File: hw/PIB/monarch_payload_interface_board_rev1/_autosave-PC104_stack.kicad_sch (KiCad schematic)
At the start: 19 parts, among them U1 Payload, U10 AD7124-8BCPZ-RL, U11 WSK06121L000FEA, U12 WSK06121L000FEA, U13 WSK06121L000FEA

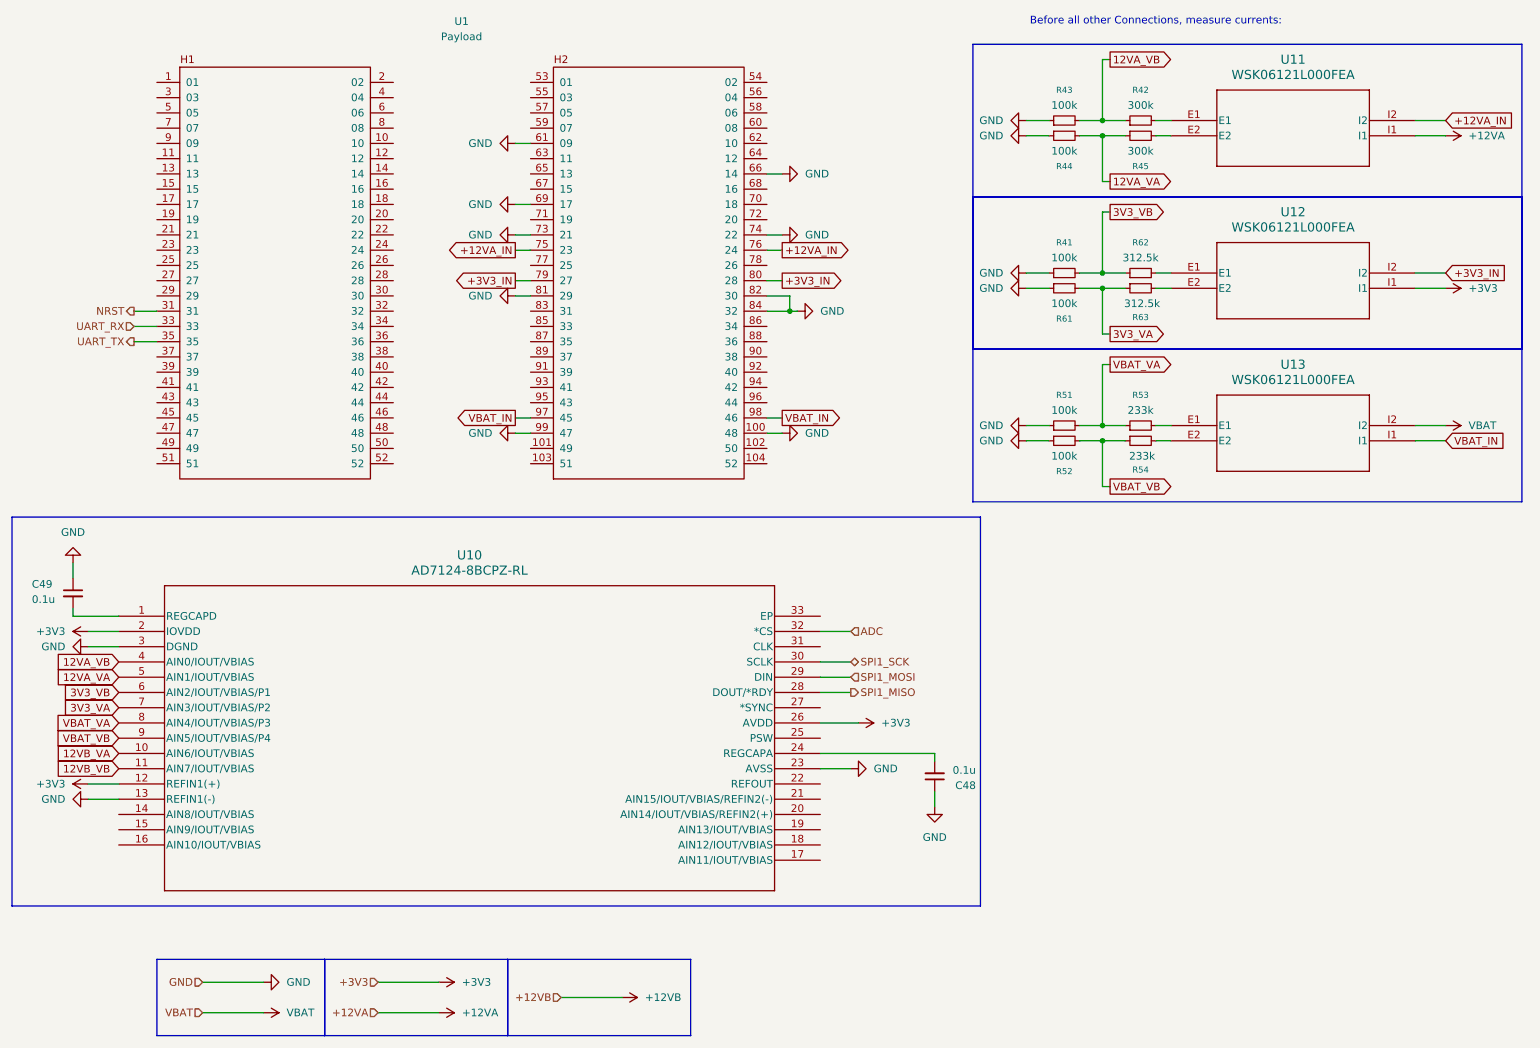
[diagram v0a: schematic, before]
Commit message: PIB Progress
Most MCU pins selected. more to come.
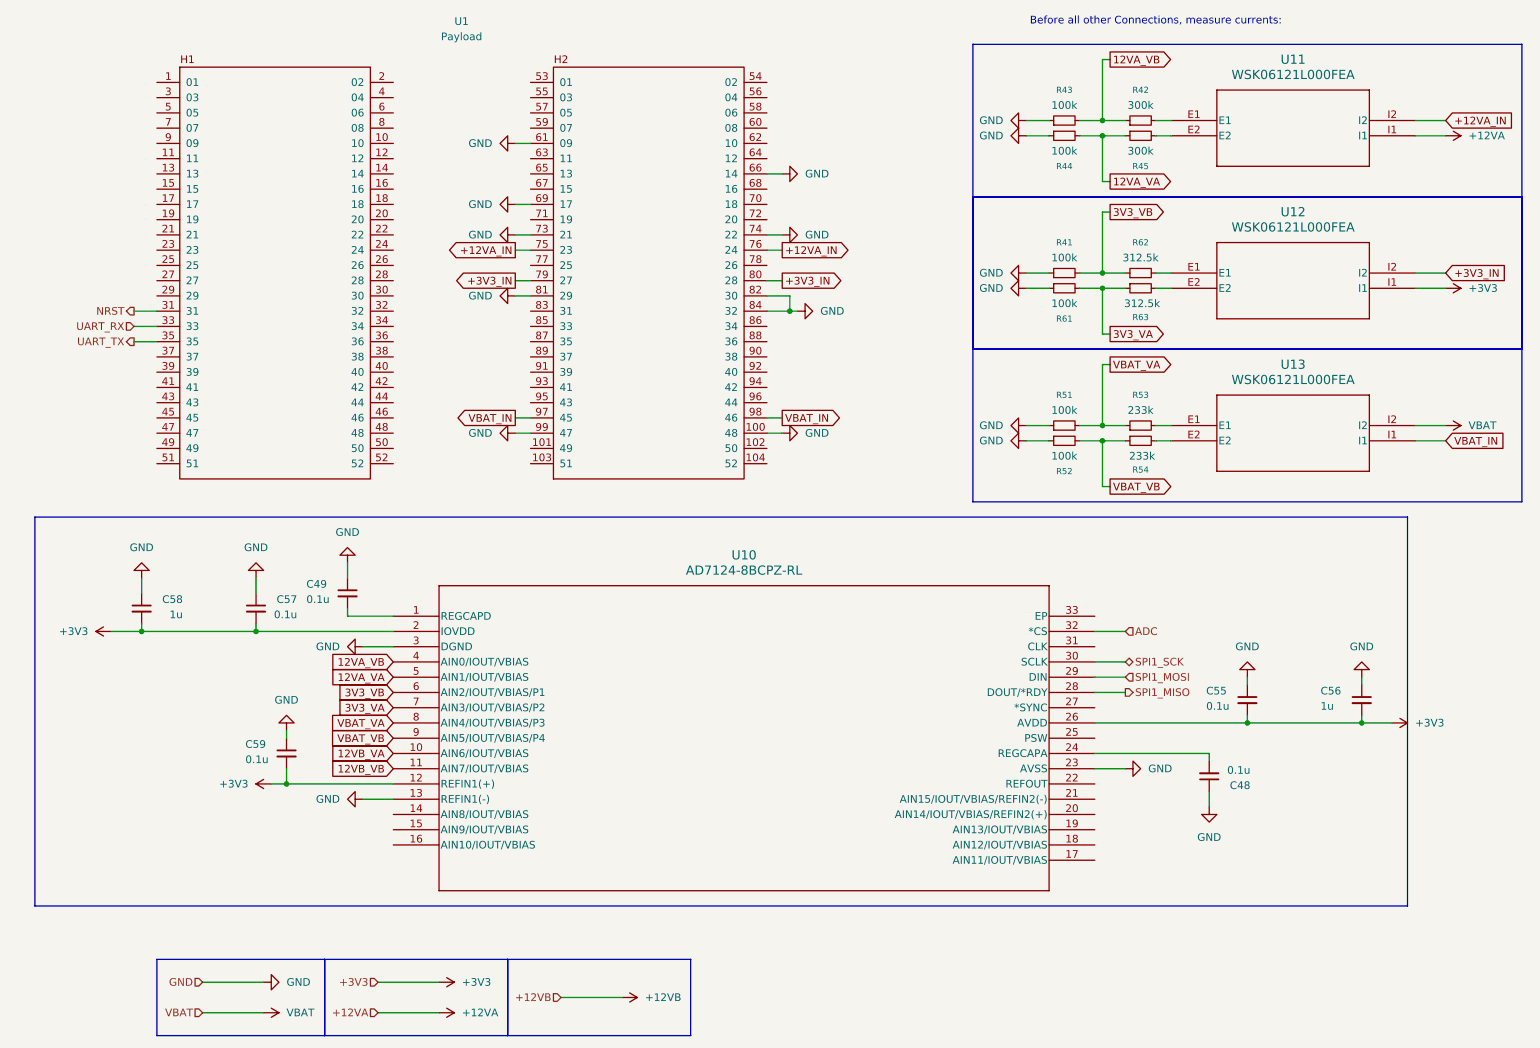
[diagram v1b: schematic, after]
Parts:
- added C55, C57, C59: 0.1u, Capacitor_SMD:C_0603_1608Metric, symbol Device:C_Small
- added C56, C58: 1u, Capacitor_SMD:C_0603_1608Metric, symbol Device:C_Small
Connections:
- net +3V3: now also C55.2, C56.2, C57.2, C58.2, C59.2
- net GND: now also C55.1, C56.1, C57.1, C58.1, C59.1
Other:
- moved on the sheet: C48, C49, U10
